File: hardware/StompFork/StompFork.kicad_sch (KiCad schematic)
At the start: 32 parts, among them J1 Conn_01x02_Socket, J2 Input, J3 Direct Output, J4 Buffered Output 1, J5 Buffered Output 2, U1 TL074

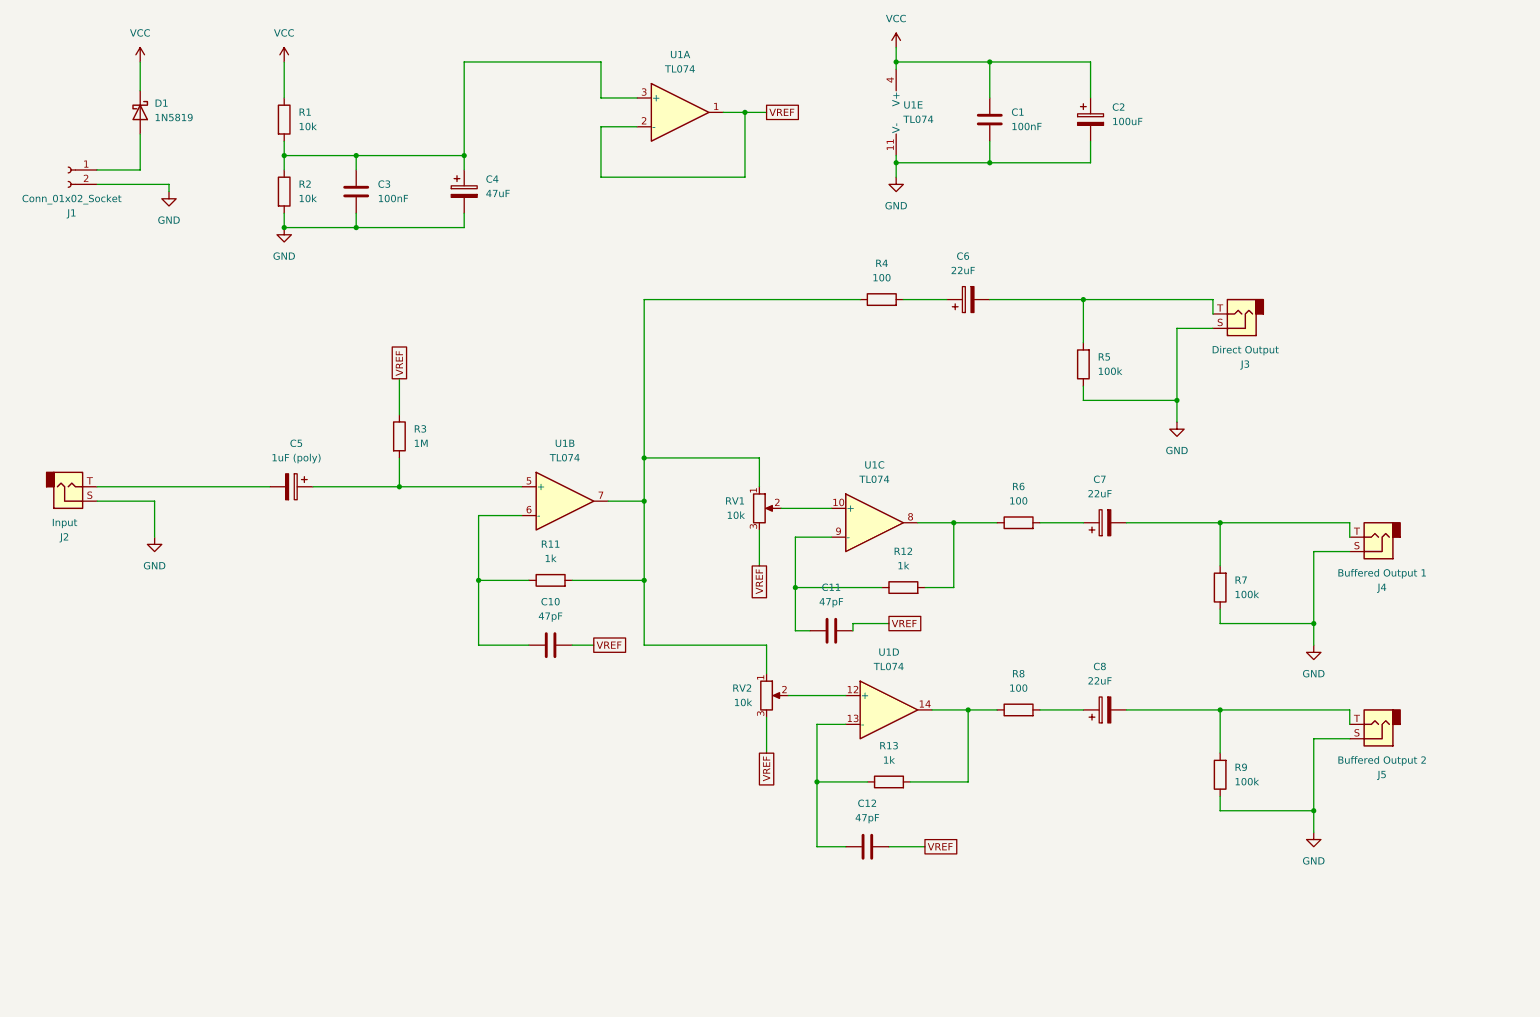
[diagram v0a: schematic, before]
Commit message: Polish schematic
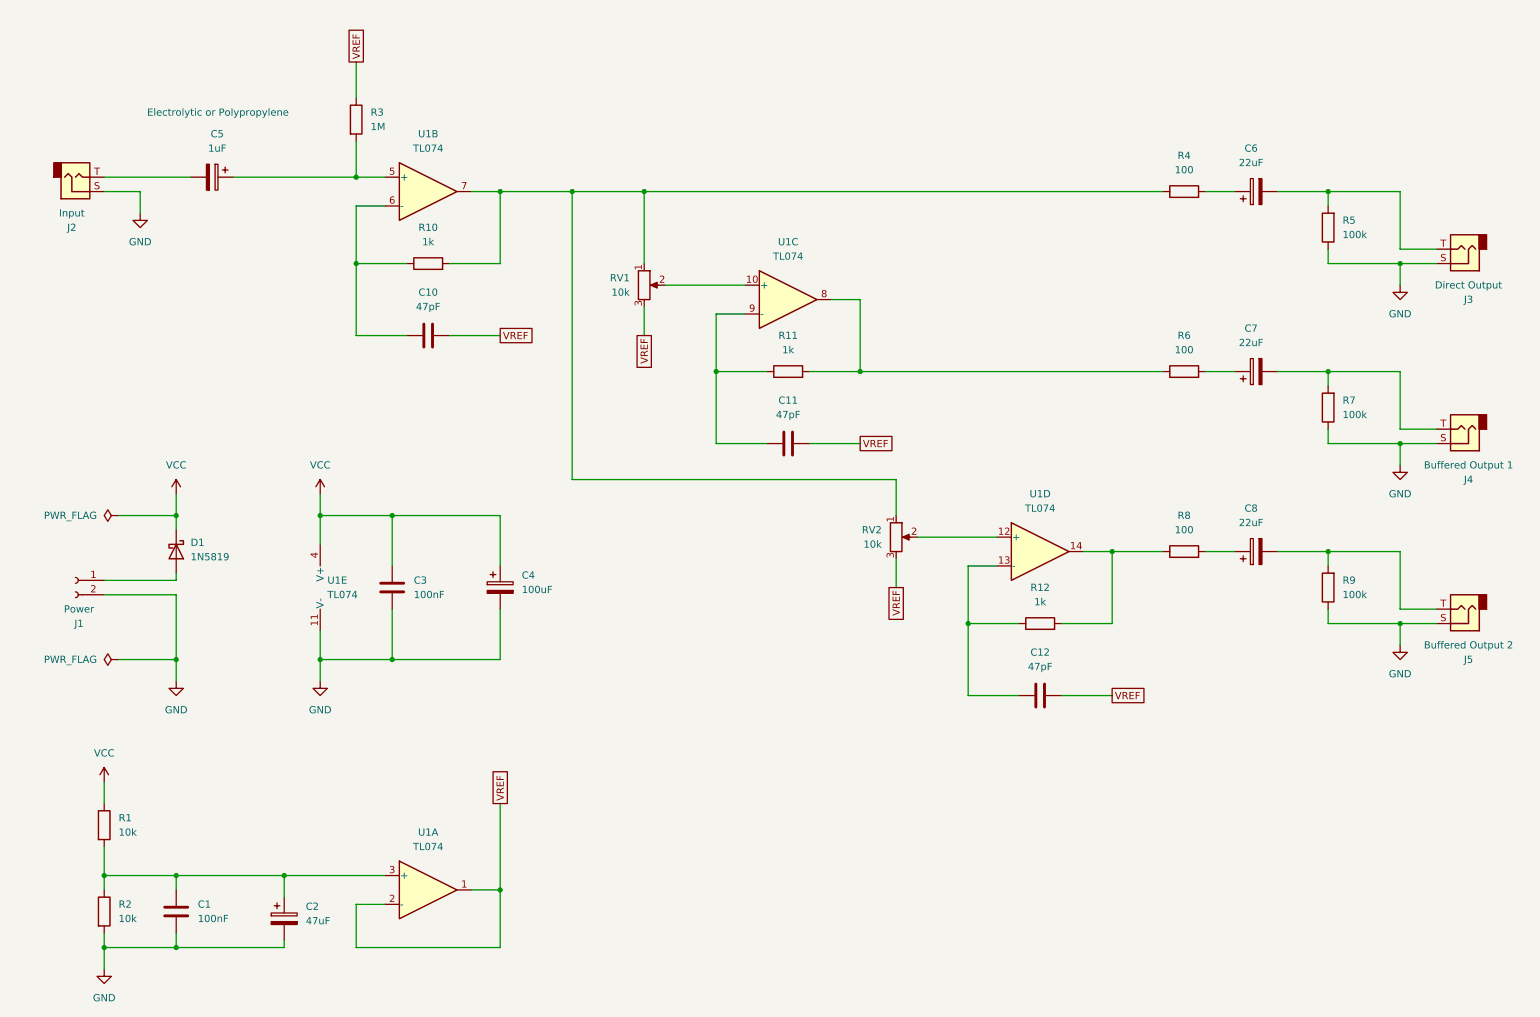
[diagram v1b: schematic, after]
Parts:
- removed C4: 47uF, symbol Device:C_Polarized
- added C2: 47uF, symbol Device:C_Polarized
- C5: value 1uF (poly) -> 1uF
- J1: value Conn_01x02_Socket -> Power
- renumbered C3 to C1, C1 to C3, C2 to C4, R11 to R10, R12 to R11, R13 to R12
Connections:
- net GND: now also C2.2
- net at C1.1, R1.2, R2.1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: now also C2.1
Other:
- moved on the sheet: C1, C10, C11, C12, C3, C4, C5, C6, C7, C8, D1, J1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
